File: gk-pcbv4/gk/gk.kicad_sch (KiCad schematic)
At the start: 19 parts

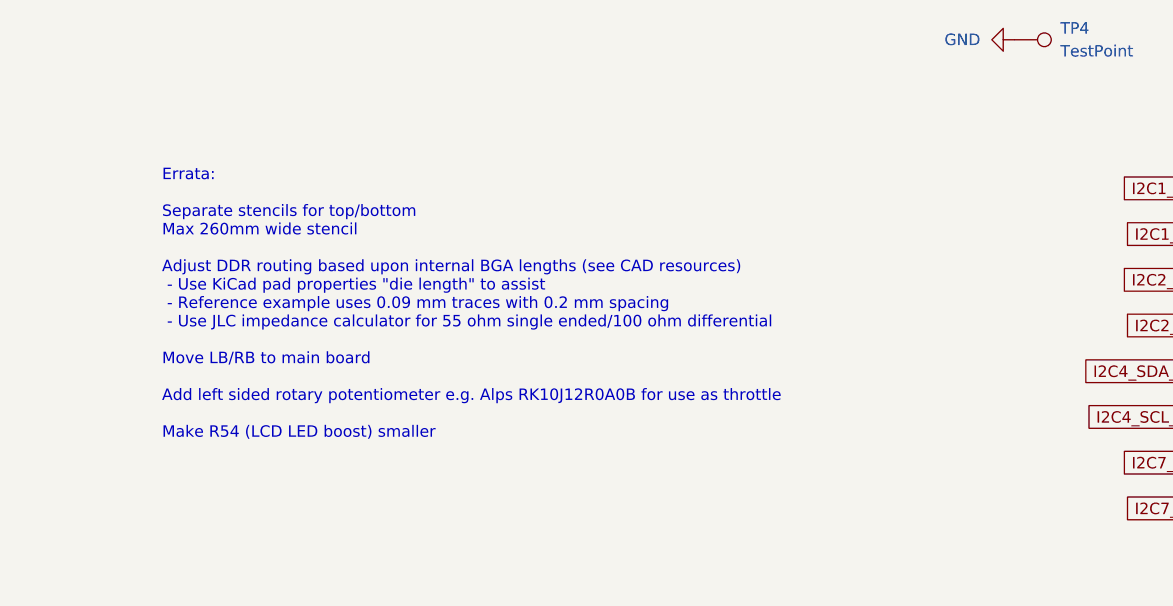
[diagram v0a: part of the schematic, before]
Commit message: Add throttle control
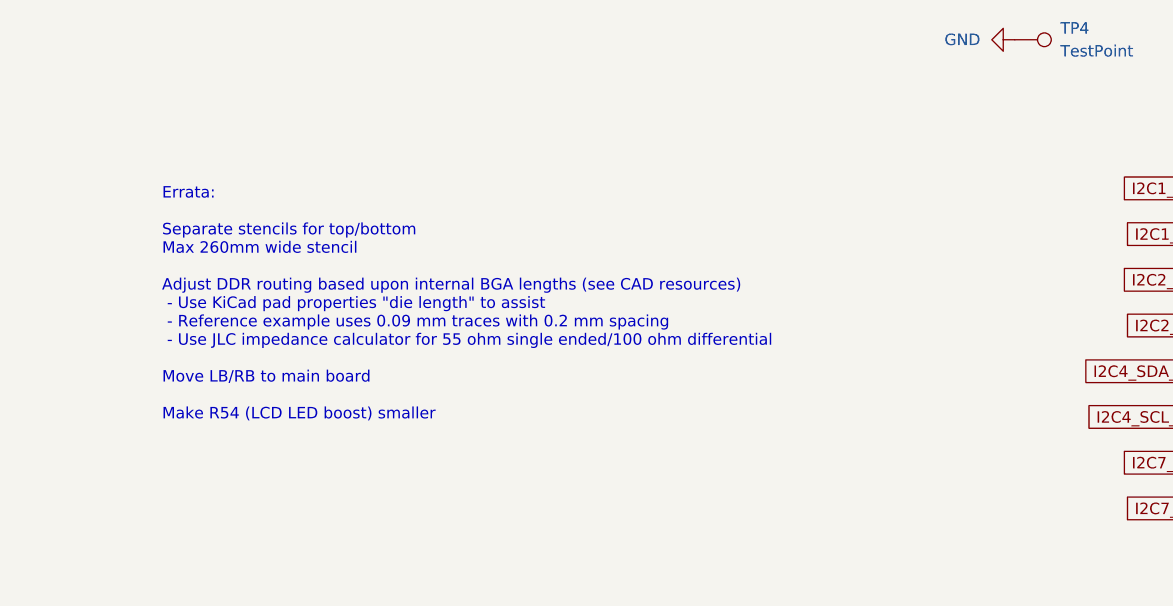
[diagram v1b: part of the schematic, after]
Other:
- note added: "Errata: Separate stencils for top/bottom Max 260mm wide stencil Adjust DDR routing based upon internal BGA lengths (see CAD resources) - Use KiCad pad properties "die length" to assist - Reference example uses 0.09 mm traces with 0.2 mm spacing - Use JLC impedance calculator for 55 ohm single ended/100 ohm differential Move LB/RB to main board Make R54 (LCD LED boost) smaller"
- note removed: "Errata: Separate stencils for top/bottom Max 260mm wide stencil Adjust DDR routing based upon internal BGA lengths (see CAD resources) - Use KiCad pad properties "die length" to assist - Reference example uses 0.09 mm traces with 0.2 mm spacing - Use JLC impedance calculator for 55 ohm single ended/100 ohm differential Move LB/RB to main board Add left sided rotary potentiometer e.g. Alps RK10J12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"
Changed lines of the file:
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@@
 		)
 	)
-	(text "Errata:\n\nSeparate stencils for top/bottom\nMax 260mm wide stencil\n\nAdjust DDR routing based upon internal BGA lengths (see CAD resources)\n - Use KiCad pad properties \"die length\" to assist\n - Reference example uses 0.09 mm traces with 0.2 mm spacing\n - Use JLC impedance calculator for 55 ohm single ended/100 ohm differential\n\nMove LB/RB to main board\n\nAdd left sided rotary potentiometer e.g. Alps RK10J12R0A0B for use as throttle\n\nMake R54 (LCD LED boost) smaller\n\n"
+	(text "Errata:\n\nSeparate stencils for top/bottom\nMax 260mm wide stencil\n\nAdjust DDR routing based upon internal BGA lengths (see CAD resources)\n - Use KiCad pad properties \"die length\" to assist\n - Reference example uses 0.09 mm traces with 0.2 mm spacing\n - Use JLC impedance calculator for 55 ohm single ended/100 ohm differential\n\nMove LB/RB to main board\n\nMake R54 (LCD LED boost) smaller\n\n"
 		(exclude_from_sim no)
 		(at 104.648 80.01 0)
